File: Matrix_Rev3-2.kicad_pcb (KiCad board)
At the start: 2 copper layers, 34 parts, among them SW1 DPST, SW10 DPST, SW11 DPST, SW12 DPST, SW13 DPST, SW14 DPST, SW15 DPST, SW16 DPST, SW2 DPST, SW3 DPST, SW4 DPST, SW5 DPST, SW6 DPST, SW7 DPST, SW8 DPST, SW9 DPST

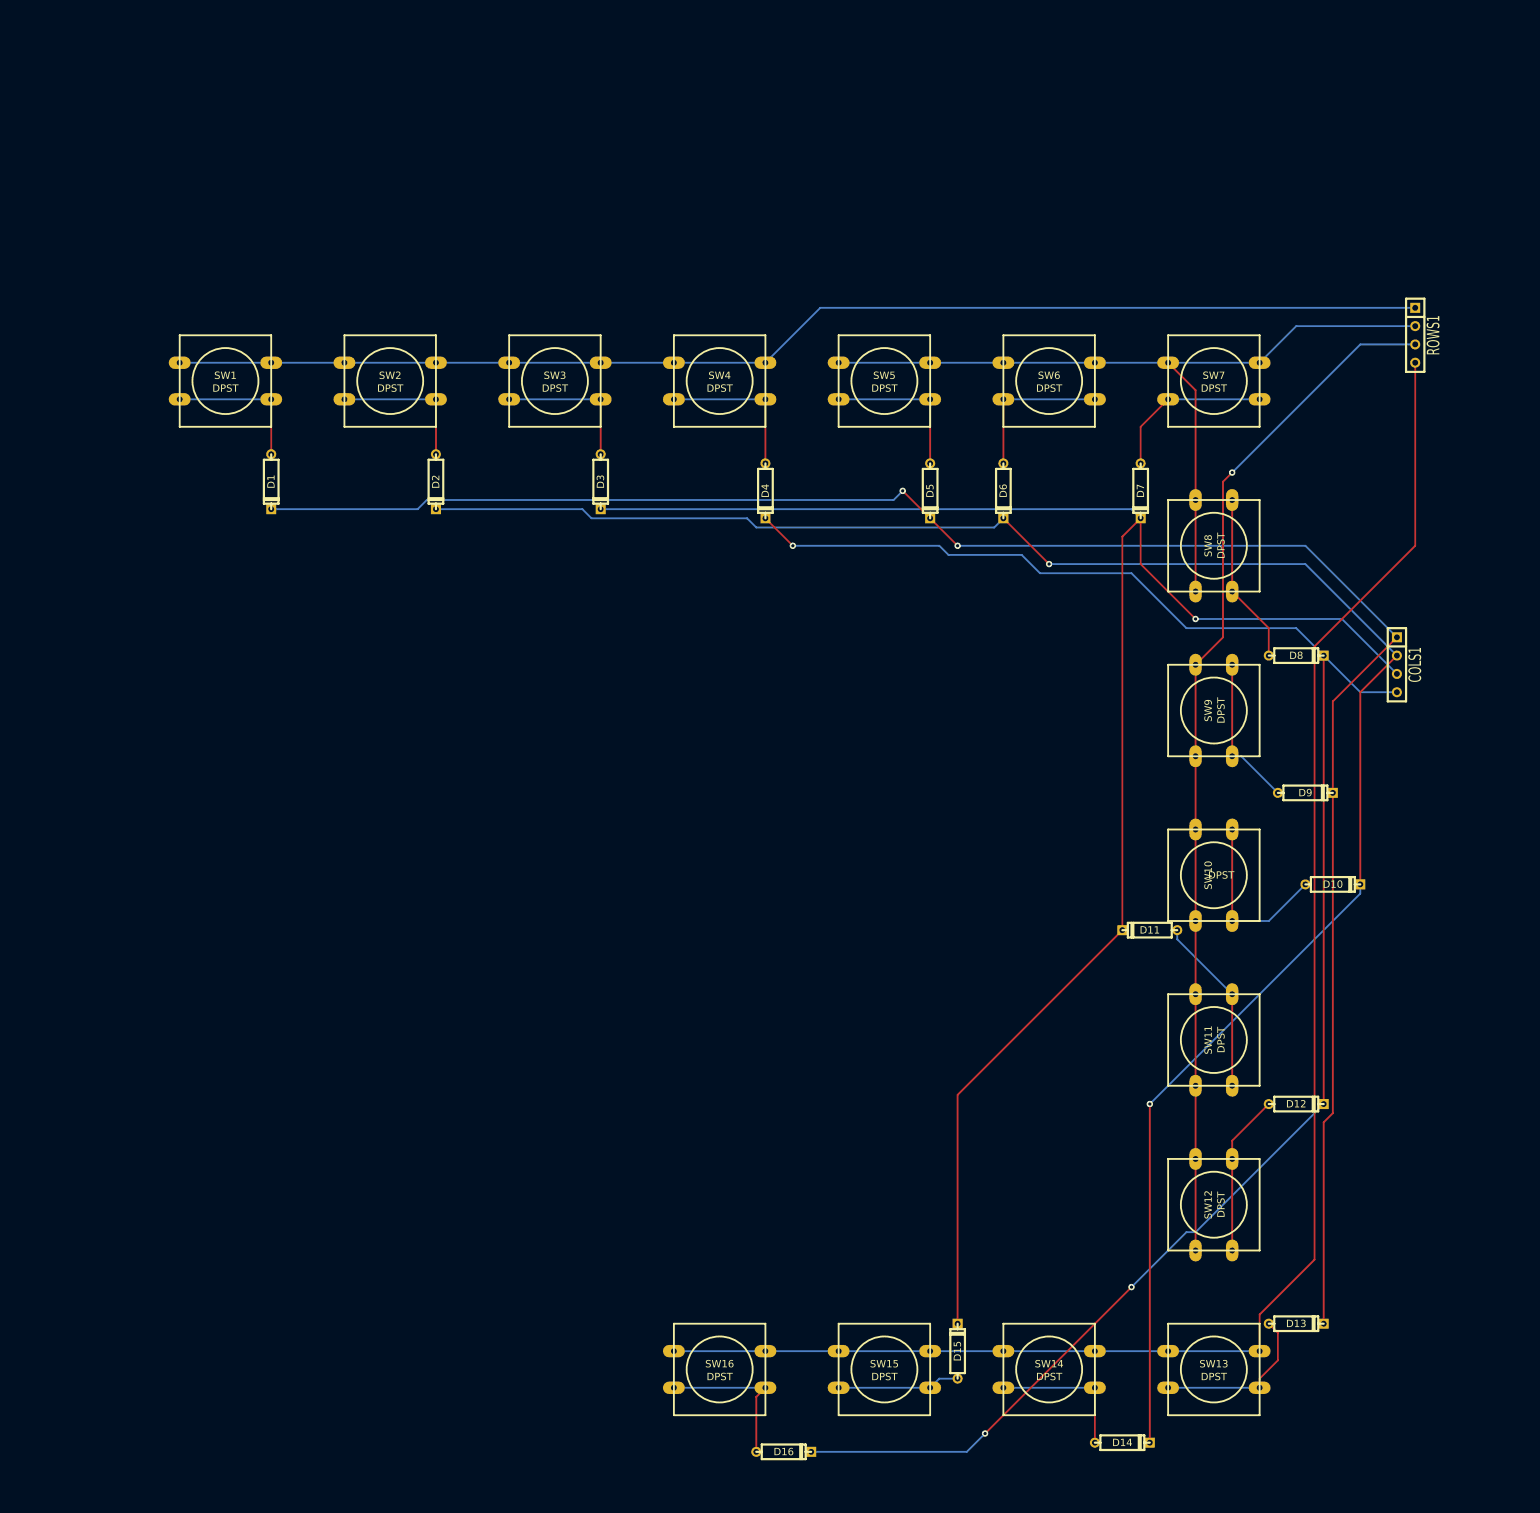
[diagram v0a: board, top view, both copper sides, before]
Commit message: New libary files etc
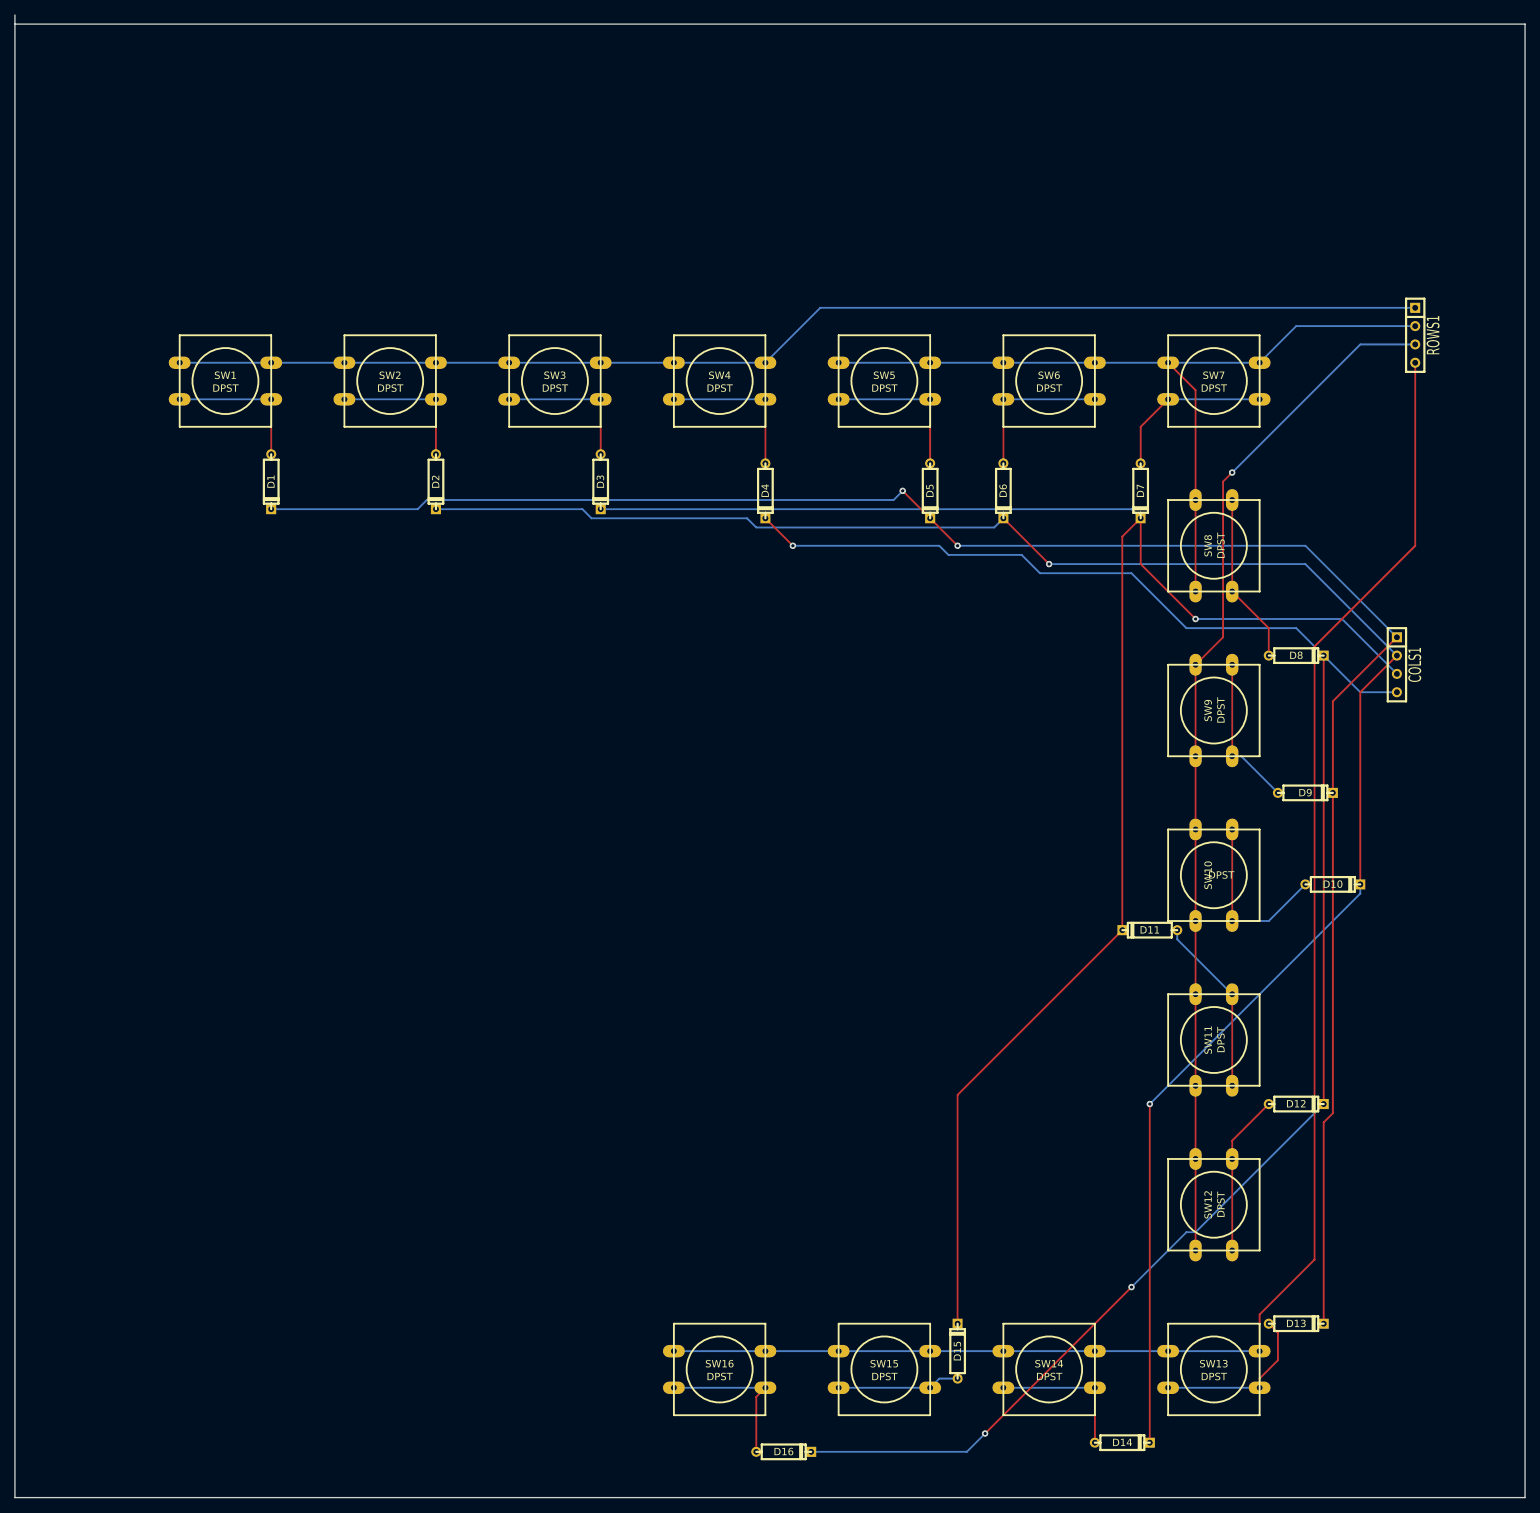
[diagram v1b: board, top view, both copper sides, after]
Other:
- board outline added: 209.6 x 205.7 mm
